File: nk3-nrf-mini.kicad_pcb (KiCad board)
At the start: 4 copper layers, 16.4 x 11.1 mm, 35 parts, among them J1 USB_A, U1 nRF52840, U3 quad_serial_flash, U5 SE050, Y1 TAXM32M4ZFBCCT2T

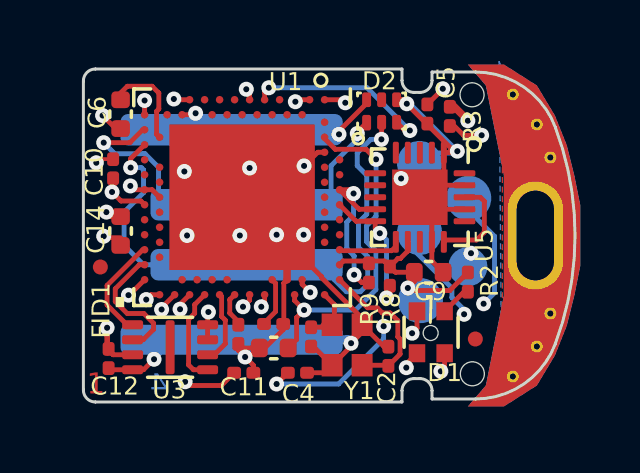
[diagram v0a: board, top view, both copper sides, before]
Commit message: nk3am121+122
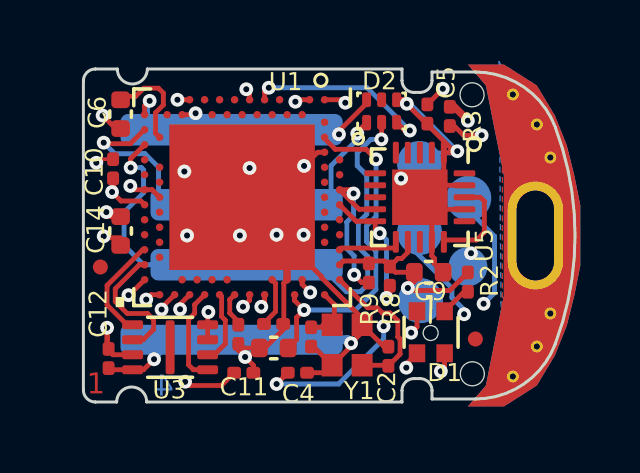
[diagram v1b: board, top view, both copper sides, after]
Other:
- outline, holes or cut-outs redrawn
- net class Default removed
